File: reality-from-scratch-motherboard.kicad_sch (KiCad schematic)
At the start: 43 parts, among them IC1 ICM-42688-P, J102 TC2050-IDC, U1 RP2040, U101 W25Q128JVS, U102 USB-TYPE-C-018, U103 NCP1117-3.3_SOT223, U104 TS-1187A-B-A-B, X101 X322512MSB4SI

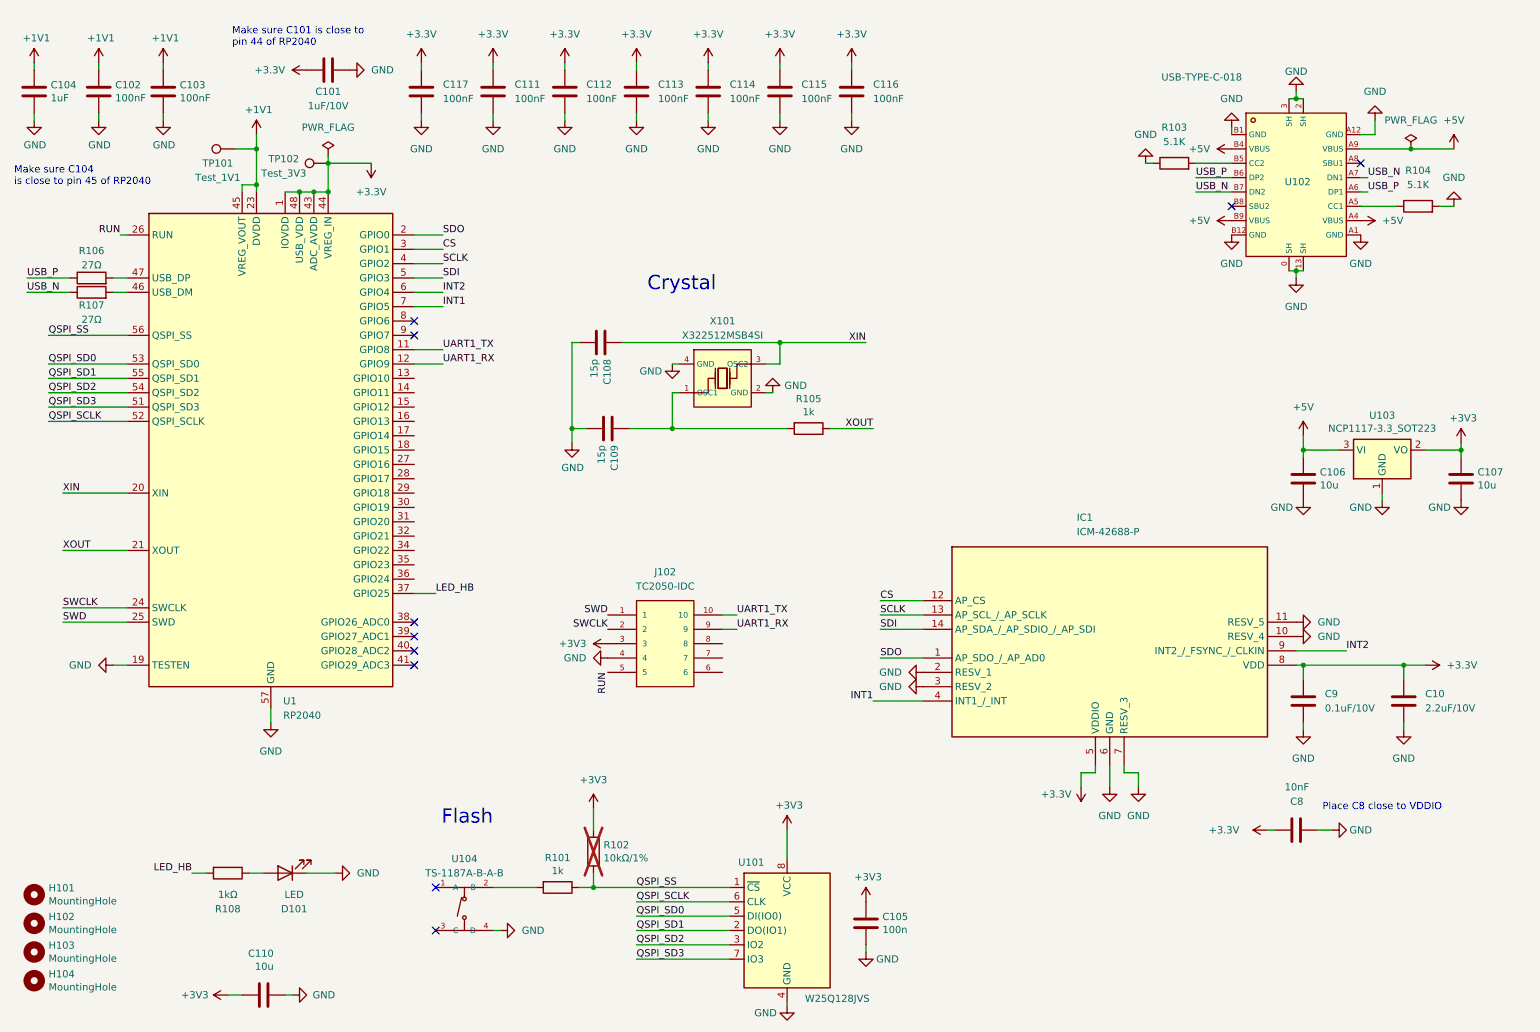
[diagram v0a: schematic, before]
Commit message: fixed MD file
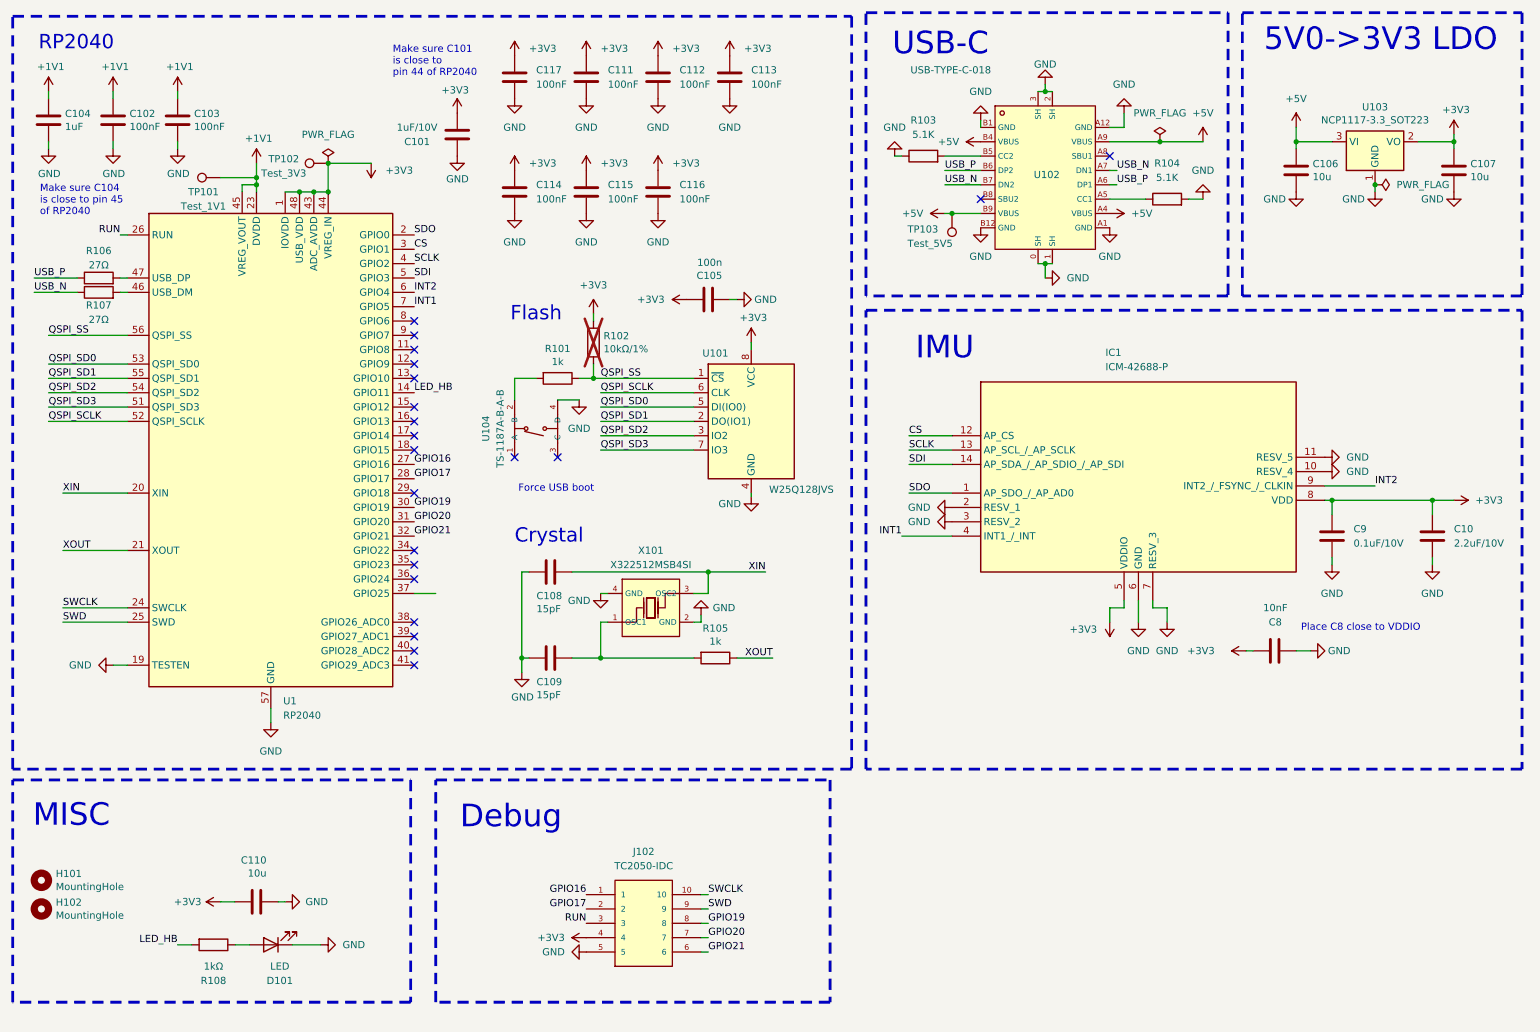
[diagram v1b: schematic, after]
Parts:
- removed H103, H104: MountingHole, MountingHole:MountingHole_2.7mm_M2.5, symbol Mechanical:MountingHole
- added TP103: Test_5V5, TestPoint:TestPoint_Pad_D1.5mm, symbol Connector:TestPoint
- C10, C101, C111, C112, C113, C114, C115, C116, C117, C8, C9, R106, R107, R108: footprint (none) -> Capacitor_SMD:C_0402_1005Metric
- C106, C107, C110: footprint Capacitor_SMD:C_0805_2012Metric -> Capacitor_SMD:C_0402_1005Metric
- C108, C109: value 15p -> 15pF
- D101: footprint (none) -> LED_SMD:LED_0603_1608Metric
- IC1: footprint IIM42352 -> footprints:IIM42352
- TP101, TP102: footprint (none) -> TestPoint:TestPoint_Pad_D1.5mm
- U102: footprint footprint:USB-C_SMD-TYPE-C-31-M-12 -> footprints:USB-C_SMD-TYPE-C-31-M-12
- U104: footprint footprint:SW-SMD_4P-L5.1-W5.1-P3.70-LS6.5-TL-2 -> footprints:SW-SMD_4P-L5.1-W5.1-P3.70-LS6.5-TL-2
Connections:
- net +3.3V is gone; now on net +3V3: C10.1, C101.1, C111.1, C112.1, C113.1, C114.1, C115.1, C116.1, C117.1, C8.1, C9.1, IC1.5 (VDDIO), IC1.8 (VDD), TP102.1, U1.1 (IOVDD), U1.10 (IOVDD), U1.22 (IOVDD), U1.33 (IOVDD), U1.42 (IOVDD), U1.43 (ADC_AVDD), U1.44 (VREG_IN), U1.48 (USB_VDD), U1.49 (IOVDD)
- net +3V3: now also J102.4; no longer J102.3
- net +5V: now also TP103.1
- net GND: now also J102.5, U102.1 (SH); no longer J102.4, U102.13 (SH)
- net LED_HB: now also U1.14 (GPIO11); no longer U1.37 (GPIO25)
- net RUN: now also J102.3; no longer J102.5
- net SWCLK: now also J102.10; no longer J102.2
- net SWD: now also J102.9; no longer J102.1
- net GPIO16: now reaches U1.27 (GPIO16)
- net GPIO16: now also J102.1
- net GPIO17: now reaches U1.28 (GPIO17)
- net GPIO17: now also J102.2
- net GPIO19: now reaches U1.30 (GPIO19)
- net GPIO19: now also J102.8
- net GPIO20: now reaches U1.31 (GPIO20)
- net GPIO20: now also J102.7
- net GPIO21: now reaches U1.32 (GPIO21)
- net GPIO21: now also J102.6
- net UART1_RX: no longer names the net of U1.12 (GPIO9)
- net UART1_RX: no longer J102.9
- net UART1_TX: no longer names the net of U1.11 (GPIO8)
- net UART1_TX: no longer J102.10
- no-connect marks 10 -> 21
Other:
- note added: "5V0->3V3 LDO"
- note added: "Debug"
- note added: "Force USB boot"
- note added: "IMU"
- note added: "MISC"
- note added: "RP2040"
- note added: "USB-C"
- moved on the sheet: C10, C101, C102, C103, C104, C105, C106, C107, C108, C109, C110, C111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
